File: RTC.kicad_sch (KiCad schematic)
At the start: 7 parts, among them P16 CONN_4, U47 M6242, X1 RTC_OSC

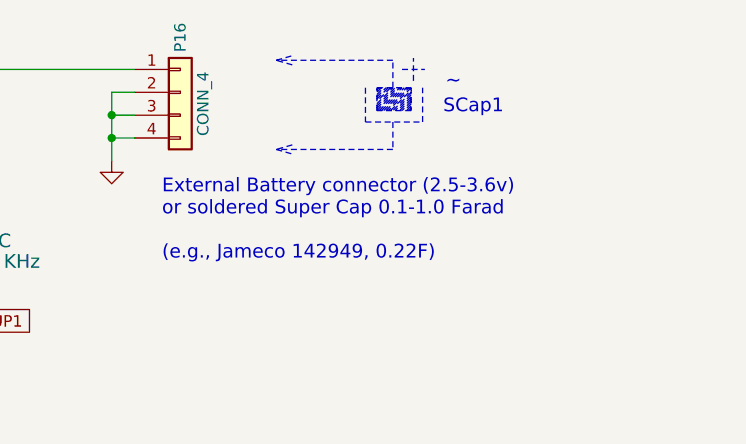
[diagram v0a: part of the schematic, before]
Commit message: minor schematic clean up
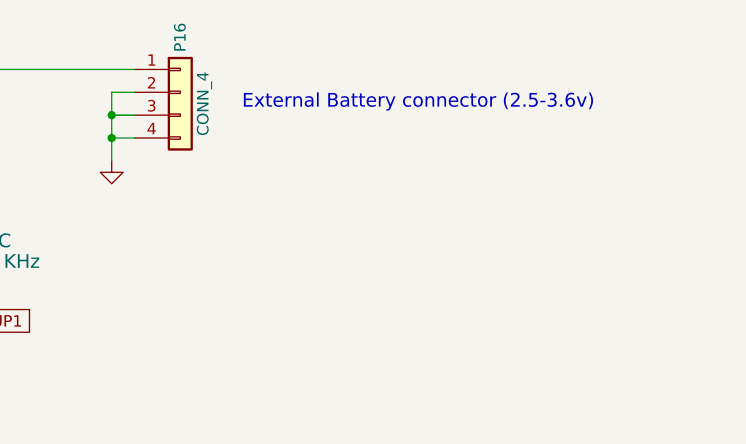
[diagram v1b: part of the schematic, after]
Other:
- note added: "External Battery connector (2.5-3.6v)"
- note removed: "External Battery connector (2.5-3.6v) or soldered Super Cap 0.1-1.0 Farad (e.g., Jameco 142949, 0.22F)"
- note removed: "SCap1"
- note removed: "~"
